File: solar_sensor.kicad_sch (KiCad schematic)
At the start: 3 parts

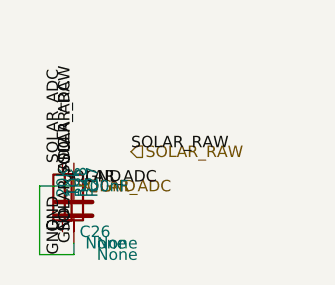
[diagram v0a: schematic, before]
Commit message: fic placer for small schemes
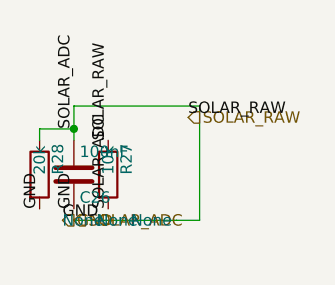
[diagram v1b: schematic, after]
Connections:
- net GND: no longer C26.1, R27.2, R28.1
- new net SOLAR_ADC: C26.1, R27.2, R28.1
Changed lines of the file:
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@@
 	(symbol
 		(lib_id "Device:C")
-		(at 17.78 19.05 0)
+		(at 17.78 15.24 0)
 		(unit 1)
 		(exclude_from_sim no)
@@
 		(fields_autoplaced no)
 		(property "Reference" "C26"
-			(at 18.415 21.59 0.0000)
+			(at 18.415 17.78 0.0000)
 			(effects
 				(font
@@
 		)
 		(property "Value" "100nF"
-			(at 18.415 16.51 0.0000)
+			(at 18.415 12.7 0.0000)
 			(effects
 				(font
@@
 		)
 		(property "mirror" "None"
-			(at 20.32 24.1299 0)
+			(at 20.32 20.3199 0)
 			(effects
 				(font
@@
 		(instances
 			(project "Untitled"
-				(path "/0db772c6-c8f2-4d81-8602-14e856cc1f5d"
+				(path "/1fbe9de3-9289-44a8-9734-4d68a48c9c9d"
 					(reference "C26")
 					(unit 1)
@@
 	(symbol
 		(lib_id "Device:R")
-		(at 17.78 17.78 0)
+		(at 21.59 15.24 0)
 		(unit 1)
 		(exclude_from_sim no)
@@
 		(fields_autoplaced no)
 		(property "Reference" "R27"
-			(at 19.812 17.78 90)
+			(at 23.622 15.24 90)
 			(effects
 				(font
@@
 		)
 		(property "Value" "10k"
-			(at 17.78 17.78 90)
+			(at 21.59 15.24 90)
 			(effects
 				(font
@@
 		)
 		(property "mirror" "None"
-			(at 20.32 22.8599 0)
+			(at 24.13 20.3199 0)
 			(effects
 				(font
@@
 		(instances
 			(project "Untitled"
-				(path "/0db772c6-c8f2-4d81-8602-14e856cc1f5d"
+				(path "/1fbe9de3-9289-44a8-9734-4d68a48c9c9d"
 					(reference "R27")
 					(unit 1)
@@
 	(symbol
 		(lib_id "Device:R")
-		(at 16.51 17.78 0)
+		(at 13.97 15.24 0)
 		(unit 1)
 		(exclude_from_sim no)
@@
 		(fields_autoplaced no)
 		(property "Reference" "R28"
-			(at 18.542 17.78 90)
+			(at 16.002 15.24 90)
 			(effects
 				(font
@@
 		)
 		(property "Value" "20k"
-			(at 16.51 17.78 90)
+			(at 13.97 15.24 90)
 			(effects
 				(font
@@
 		)
 		(property "mirror" "None"
-			(at 19.05 22.8599 0)
+			(at 16.51 20.3199 0)
 			(effects
 				(font
@@
 		(instances
 			(project "Untitled"
-				(path "/0db772c6-c8f2-4d81-8602-14e856cc1f5d"
+				(path "/1fbe9de3-9289-44a8-9734-4d68a48c9c9d"
 					(reference "R28")
 					(unit 1)
@@
 	(wire
 		(pts
-			(xy 17.78 22.86) (xy 17.78 24.13)
-		)
-		(stroke
-			(width 0)
-			(type default)
-		)
-	)
-	(wire
-		(pts
-			(xy 17.78 24.13) (xy 13.97 24.13)
-		)
-		(stroke
-			(width 0)
-			(type default)
-		)
-	)
-	(wire
-		(pts
-			(xy 13.97 24.13) (xy 13.97 16.51)
-		)
-		(stroke
-			(width 0)
-			(type default)
-		)
-	)
-	(wire
-		(pts
-			(xy 13.97 16.51) (xy 19.05 16.51)
-		)
-		(stroke
-			(width 0)
-			(type default)
-		)
+			(xy 13.97 11.43) (xy 13.97 10.16)
+		)
+		(stroke
+			(width 0)
+			(type default)
+		)
+	)
+	(wire
+		(pts
+			(xy 13.97 10.16) (xy 17.78 10.16)
+		)
+		(stroke
+			(width 0)
+			(type default)
+		)
+	)
+	(wire
+		(pts
+			(xy 17.78 10.16) (xy 17.78 11.43)
+		)
+		(stroke
+			(width 0)
+			(type default)
+		)
+	)
+	(wire
+		(pts
+			(xy 17.78 20.32) (xy 29.21 20.32)
+		)
+		(stroke
+			(width 0)
+			(type default)
+		)
+	)
+	(wire
+		(pts
+			(xy 29.21 20.32) (xy 31.75 20.32)
+		)
+		(stroke
+			(width 0)
+			(type default)
+		)
+	)
+	(wire
+		(pts
+			(xy 31.75 20.32) (xy 31.75 7.62)
+		)
+		(stroke
+			(width 0)
+			(type default)
+		)
+	)
+	(wire
+		(pts
+			(xy 31.75 7.62) (xy 17.78 7.62)
+		)
+		(stroke
+			(width 0)
+			(type default)
+		)
+	)
+	(wire
+		(pts
+			(xy 17.78 7.62) (xy 17.78 10.16)
+		)
+		(stroke
+			(width 0)
+			(type default)
+		)
+	)
+	(junction
+		(at 17.78 10.16)
+		(diameter 0)
+		(color 0 0 0 0)
 	)
 	(label "GND"
-		(at 16.51 21.59 270)
+		(at 17.78 19.05 270)
 		(effects
 			(font
@@
 	)
 	(label "GND"
-		(at 17.78 22.86 270)
+		(at 16.51 20.32 180)
 		(effects
 			(font
@@
 	)
 	(label "GND"
-		(at 19.05 16.51 180)
-		(effects
-			(font
-				(size 1.27 1.27)
-			)
-			(justify left bottom)
-		)
-	)
-	(label "GND"
-		(at 16.51 24.13 270)
+		(at 13.97 19.05 270)
 		(effects
 			(font
@@
 	)
 	(label "SOLAR_RAW"
-		(at 17.78 13.97 90)
+		(at 21.59 11.43 90)
 		(effects
 			(font
@@
 	)
 	(label "SOLAR_RAW"
-		(at 24.13 12.7 180)
+		(at 30.48 8.89 180)
 		(effects
 			(font
@@
 	)
 	(label "SOLAR_ADC"
-		(at 16.51 13.97 90)
+		(at 21.59 19.05 270)
 		(effects
 			(font
@@
 	)
 	(label "SOLAR_ADC"
-		(at 17.78 15.24 90)
-		(effects
-			(font
-				(size 1.27 1.27)
-			)
-			(justify left bottom)
-		)
-	)
-	(label "SOLAR_ADC"
-		(at 16.51 16.51 0.0000)
-		(effects
-			(font
-				(size 1.27 1.27)
-			)
-			(justify left bottom)
-		)
-	)
-	(label "SOLAR_ADC"
-		(at 17.78 21.59 270)
+		(at 17.78 10.16 270)
 		(effects
 			(font
@@
 	(hierarchical_label "GND"
 		(shape input)
-		(at 19.05 16.51 180)
+		(at 16.51 20.32 180)
 		(effects
 			(font
@@
 	(hierarchical_label "SOLAR_RAW"
 		(shape input)
-		(at 24.13 12.7 180)
+		(at 30.48 8.89 180)
 		(effects
 			(font
@@
 	(hierarchical_label "SOLAR_ADC"
 		(shape input)
-		(at 16.51 16.51 0)
-		(effects
-			(font
+		(at 17.78 20.32 0)
+		(effects
+			(font
